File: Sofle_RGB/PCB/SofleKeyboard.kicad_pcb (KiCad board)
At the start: 2 copper layers, 143.4 x 111.8 mm, 97 parts, among them J1 LED, J2 4PIN, J3 OLED, J4 key leds, J5 backlight sel, J6 indicator bypass, P1 i2c_pin, P2 i2c_pin, SW1 SW_PUSH-MX_W_LED, SW10 SW_PUSH-MX_W_LED, SW11 SW_PUSH-MX_W_LED, SW12 SW_PUSH-MX_W_LED, SW13 SW_PUSH-MX_W_LED, SW14 SW_PUSH-MX_W_LED, SW15 SW_PUSH-MX_W_LED, SW16 SW_PUSH-MX_W_LED, SW17 SW_PUSH-MX_W_LED, SW18 SW_PUSH-MX_W_LED, SW19 SW_PUSH-MX_W_LED, SW2 SW_PUSH-MX_W_LED, SW20 SW_PUSH-MX_W_LED, SW21 SW_PUSH-MX_W_LED, SW22 SW_PUSH-MX_W_LED, SW23 SW_PUSH-MX_W_LED, SW24 SW_PUSH-MX_W_LED, SW25 Rotary_Encoder_Switch, SW26 SW_PUSH-MX_W_LED, SW27 SW_PUSH-MX_W_LED, SW28 SW_PUSH-MX_W_LED, SW29 SW_PUSH-MX_W_LED, SW3 SW_PUSH-MX_W_LED, SW30 SW_PUSH-MX_W_LED, SW4 SW_PUSH-MX_W_LED, SW5 SW_PUSH-MX_W_LED, SW6 SW_PUSH-MX_W_LED, SW7 SW_PUSH-MX_W_LED, SW8 SW_PUSH-MX_W_LED, SW9 SW_PUSH-MX_W_LED, U1 ProMicro

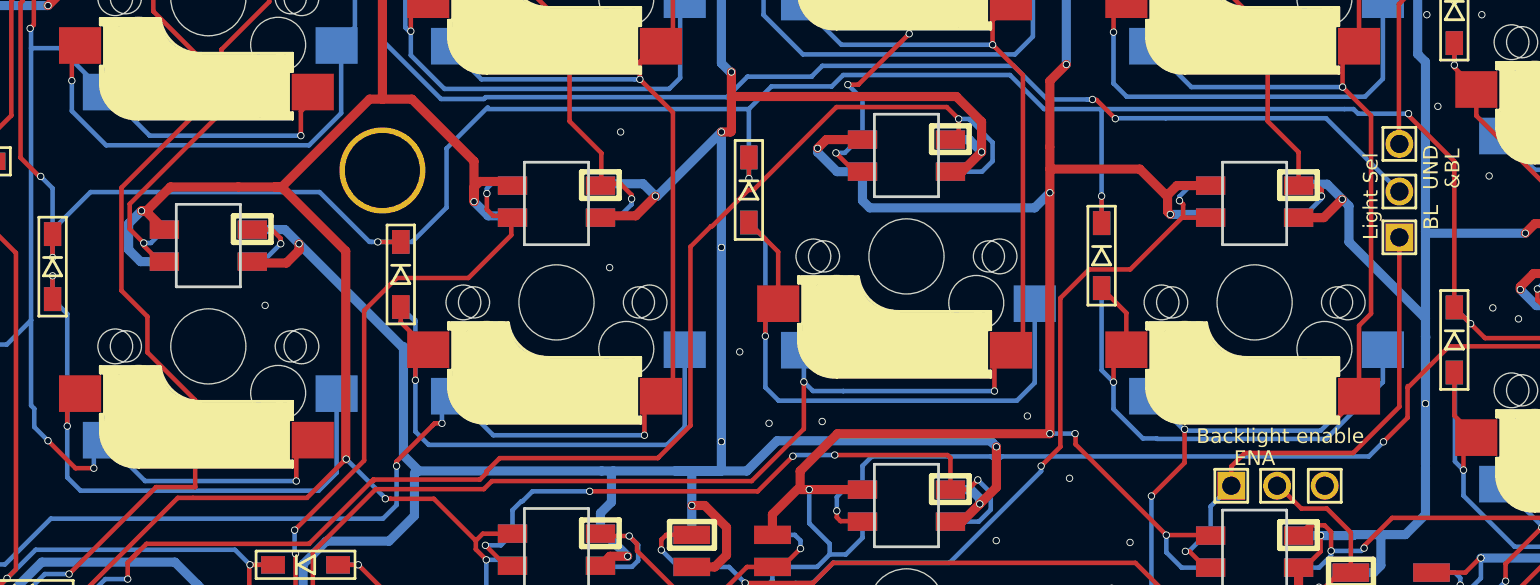
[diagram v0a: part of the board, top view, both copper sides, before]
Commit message: Address PR comments + extra cleanup
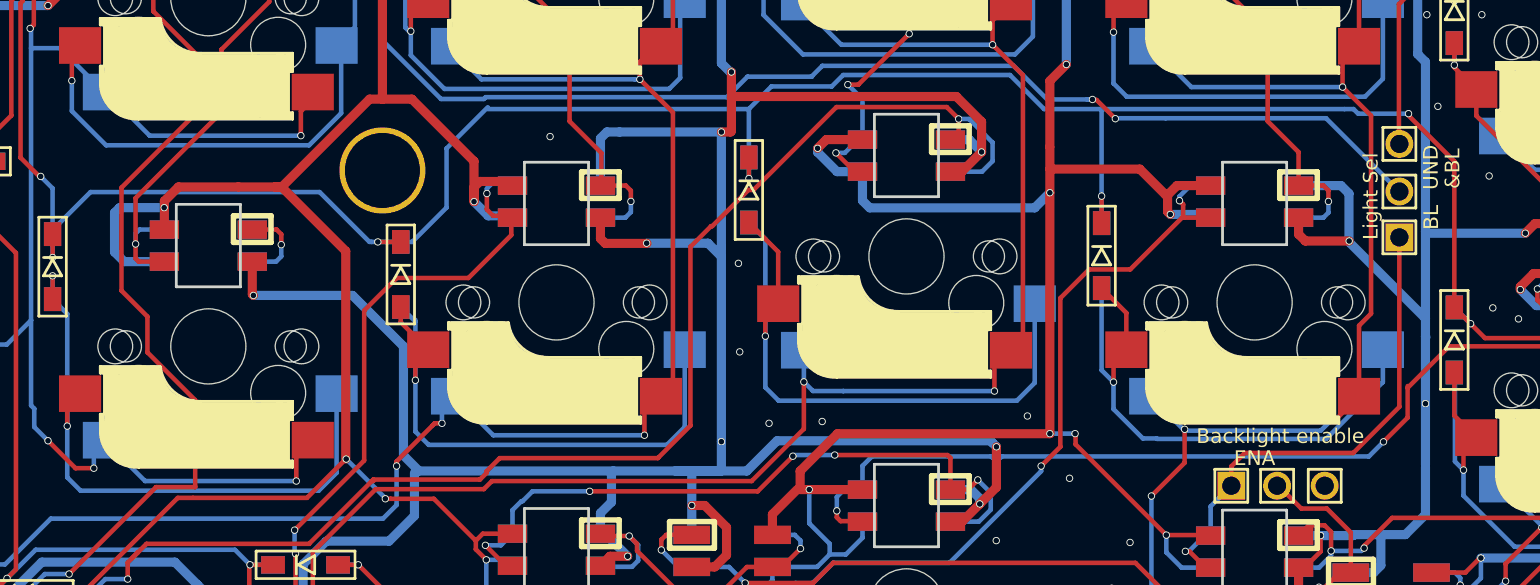
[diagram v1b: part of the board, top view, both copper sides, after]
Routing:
- net GND: track 1001.1 -> 1005.4 mm, vias 230 -> 228
- net VCC: track 928.4 -> 930.1 mm
- net Net-(SW13-Pad1): track 31.7 -> 33.2 mm
- net Net-(SW16-Pad3): track 27.3 -> 28.8 mm
- net Net-(SW19-Pad1): track 4.00 -> 5.17 mm
